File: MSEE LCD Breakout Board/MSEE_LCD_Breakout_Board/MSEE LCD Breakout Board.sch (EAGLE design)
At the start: 10 parts

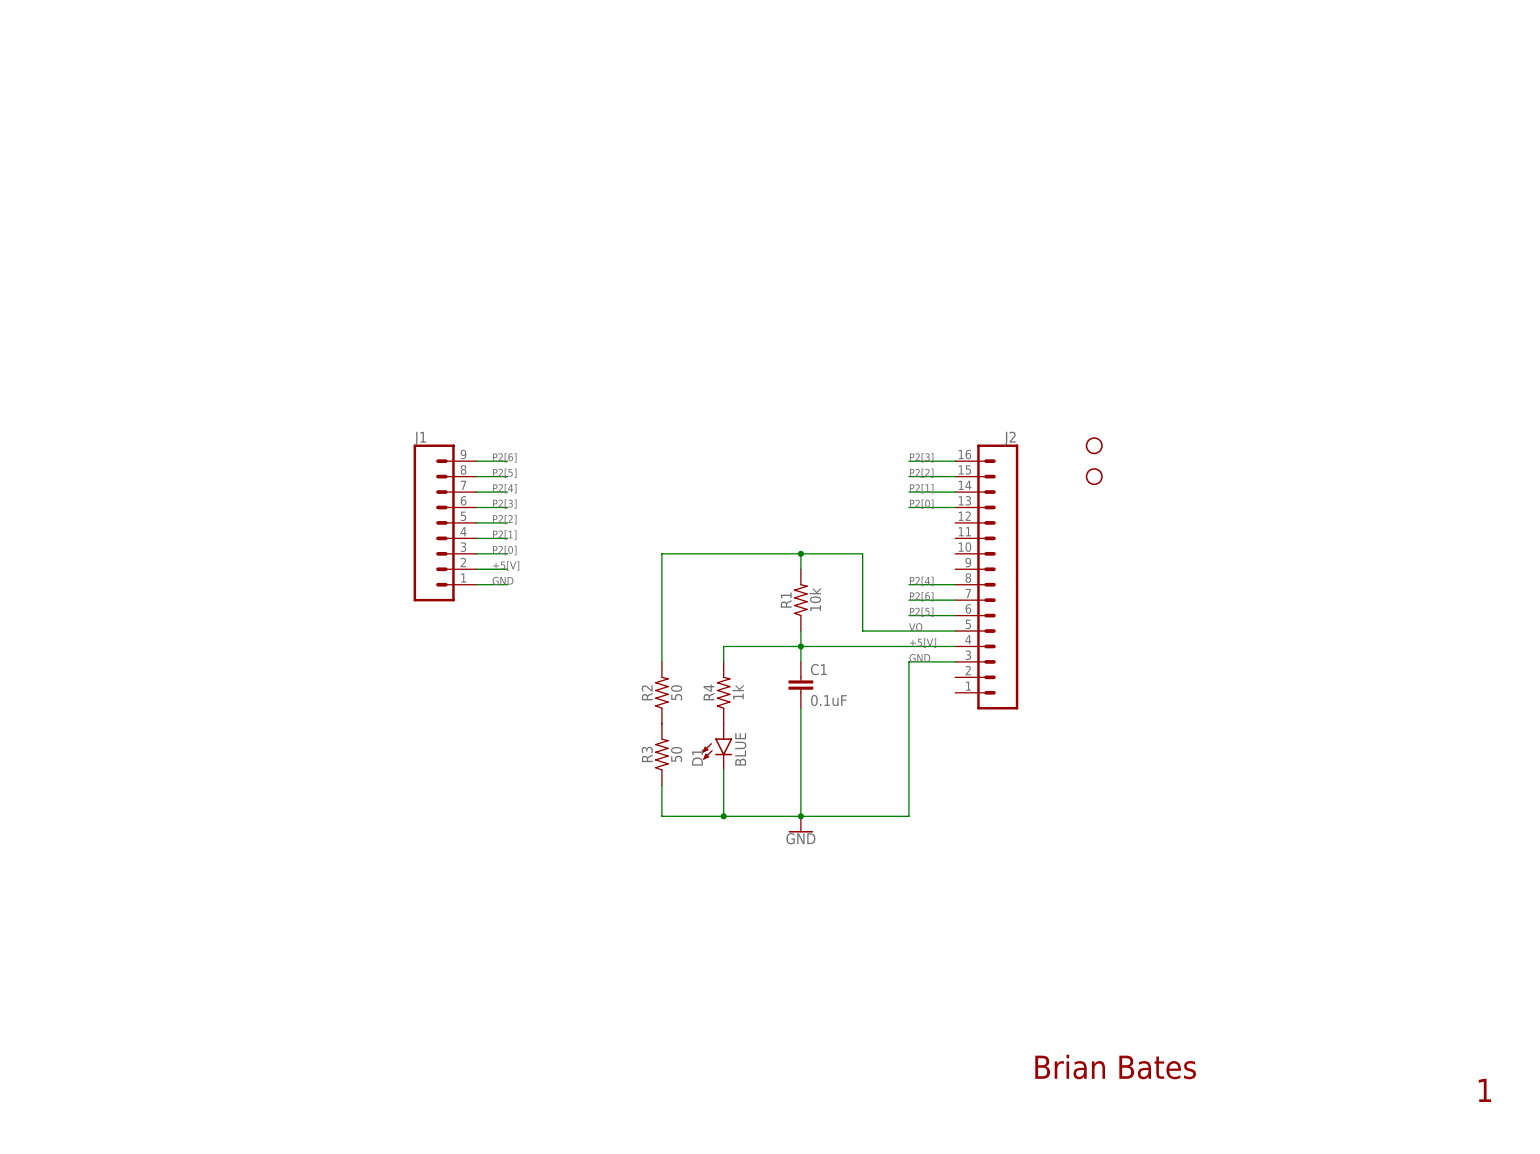
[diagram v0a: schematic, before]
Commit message: MSEE LCD Breakout Board v3
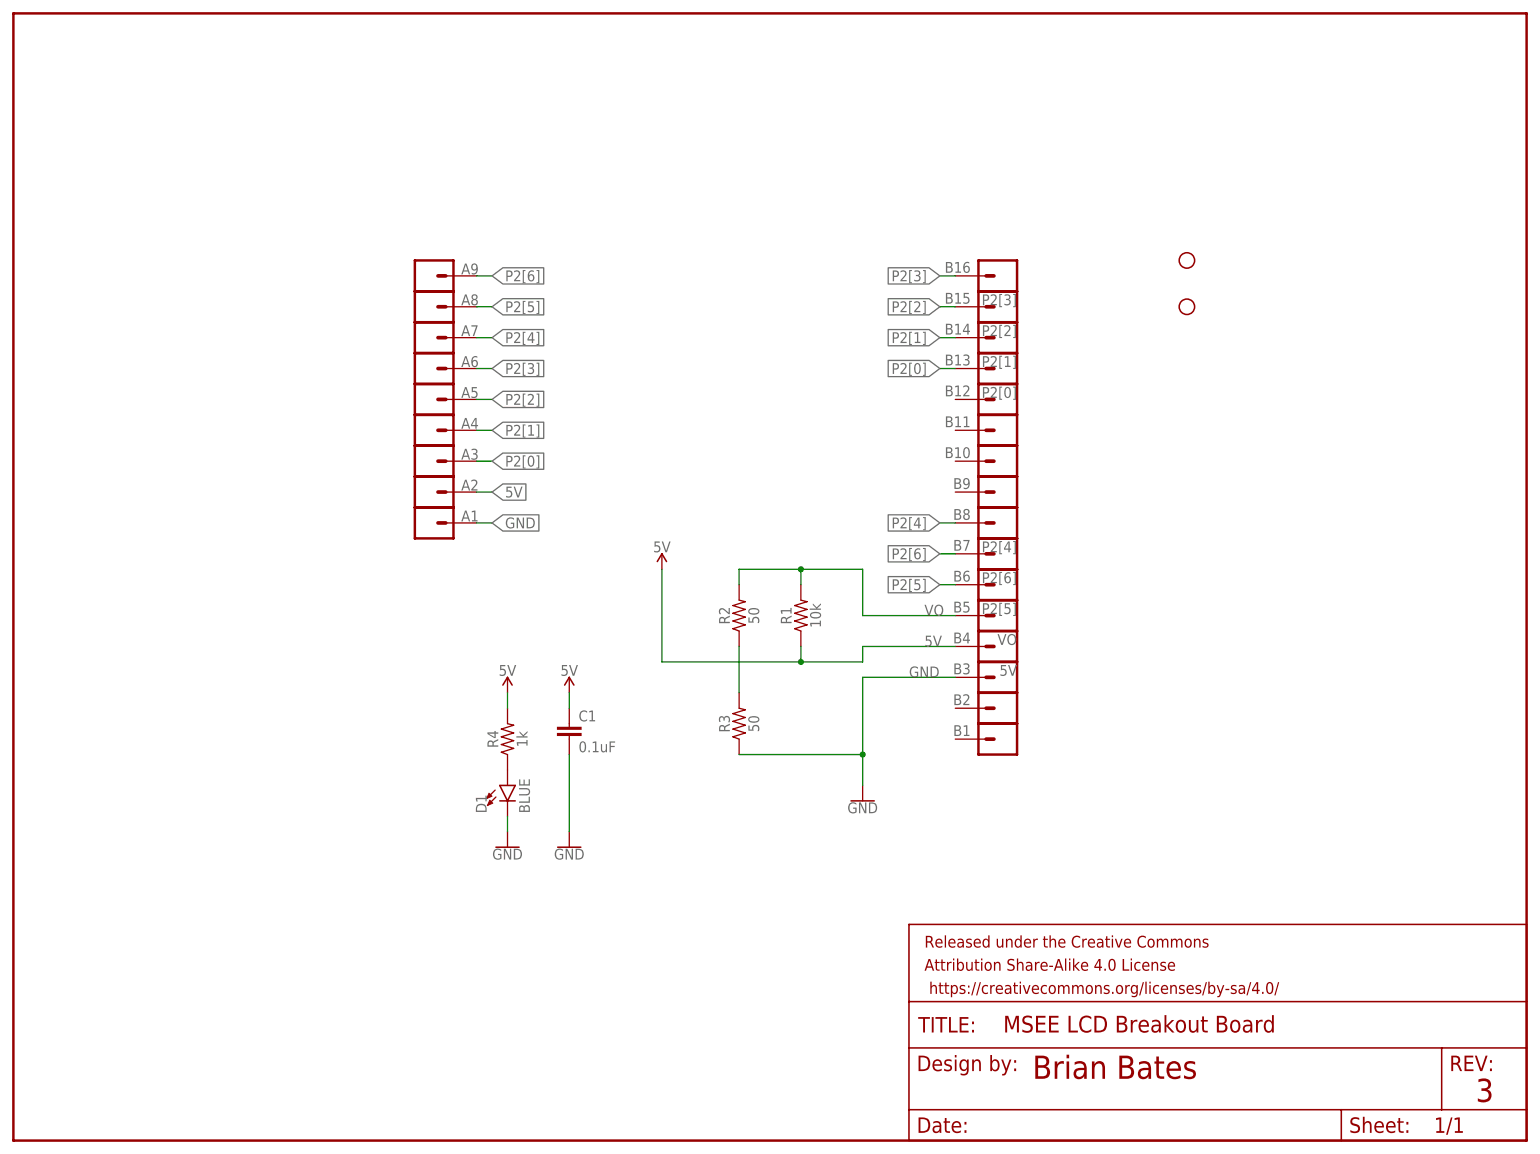
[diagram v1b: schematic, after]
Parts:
- removed J1: (no value), SparkFun-Connectors:CONN_09
- removed J2: (no value), SparkFun-Connectors:CONN_16
- added 5V: A2, SparkFun-Connectors:CONN_01PTH_LONGPAD
- added B1, B10, B11, B12, B2, B9: (no value), SparkFun-Connectors:CONN_01PTH_LONGPAD
- added B13: P2[0], SparkFun-Connectors:CONN_01PTH_LONGPAD
- added B14: P2[1], SparkFun-Connectors:CONN_01PTH_LONGPAD
- added B15: P2[2], SparkFun-Connectors:CONN_01PTH_LONGPAD
- added B16: P2[3], SparkFun-Connectors:CONN_01PTH_LONGPAD
- added B3: GND, SparkFun-Connectors:CONN_01PTH_LONGPAD
- added B4: 5V, SparkFun-Connectors:CONN_01PTH_LONGPAD
- added B5: VO, SparkFun-Connectors:CONN_01PTH_LONGPAD
- added B6: P2[5], SparkFun-Connectors:CONN_01PTH_LONGPAD
- added B7: P2[6], SparkFun-Connectors:CONN_01PTH_LONGPAD
- added B8: P2[4], SparkFun-Connectors:CONN_01PTH_LONGPAD
- added FRAME1: FRAME-LETTERNO_PACKAGE, SparkFun-Aesthetics:FRAME-LETTERNO_PACKAGE
- added GND: A1, SparkFun-Connectors:CONN_01PTH_LONGPAD
- added P2[0]: A3, SparkFun-Connectors:CONN_01PTH_LONGPAD
- added P2[1]: A4, SparkFun-Connectors:CONN_01PTH_LONGPAD
- added P2[2]: A5, SparkFun-Connectors:CONN_01PTH_LONGPAD
- added P2[3]: A6, SparkFun-Connectors:CONN_01PTH_LONGPAD
- added P2[4]: A7, SparkFun-Connectors:CONN_01PTH_LONGPAD
- added P2[5]: A8, SparkFun-Connectors:CONN_01PTH_LONGPAD
- added P2[6]: A9, SparkFun-Connectors:CONN_01PTH_LONGPAD
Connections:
- removed net +5[V]: C1.1, J1.2, J2.4, R1.1, R4.2
- new net '': C1.2
- new net 5V: 5V.1, B4.1, C1.1, R1.1, R4.2
- net GND: now also B3.1, GND.1; no longer C1.2, J1.1, J2.3
- net P2[0]: now also B13.1, P2[0].1; no longer J1.3, J2.13
- net P2[1]: now also B14.1, P2[1].1; no longer J1.4, J2.14
- net P2[2]: now also B15.1, P2[2].1; no longer J1.5, J2.15
- net P2[3]: now also B16.1, P2[3].1; no longer J1.6, J2.16
- net P2[4]: now also B8.1, P2[4].1; no longer J1.7, J2.8
- net P2[5]: now also B6.1, P2[5].1; no longer J1.8, J2.6
- net P2[6]: now also B7.1, P2[6].1; no longer J1.9, J2.7
- net VO: now also B5.1; no longer J2.5
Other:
- note added: "3"
- note removed: "1"
- moved on the sheet: C1, D1, R1, R2, R3, R4
